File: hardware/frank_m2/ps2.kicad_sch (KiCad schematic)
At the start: 14 parts

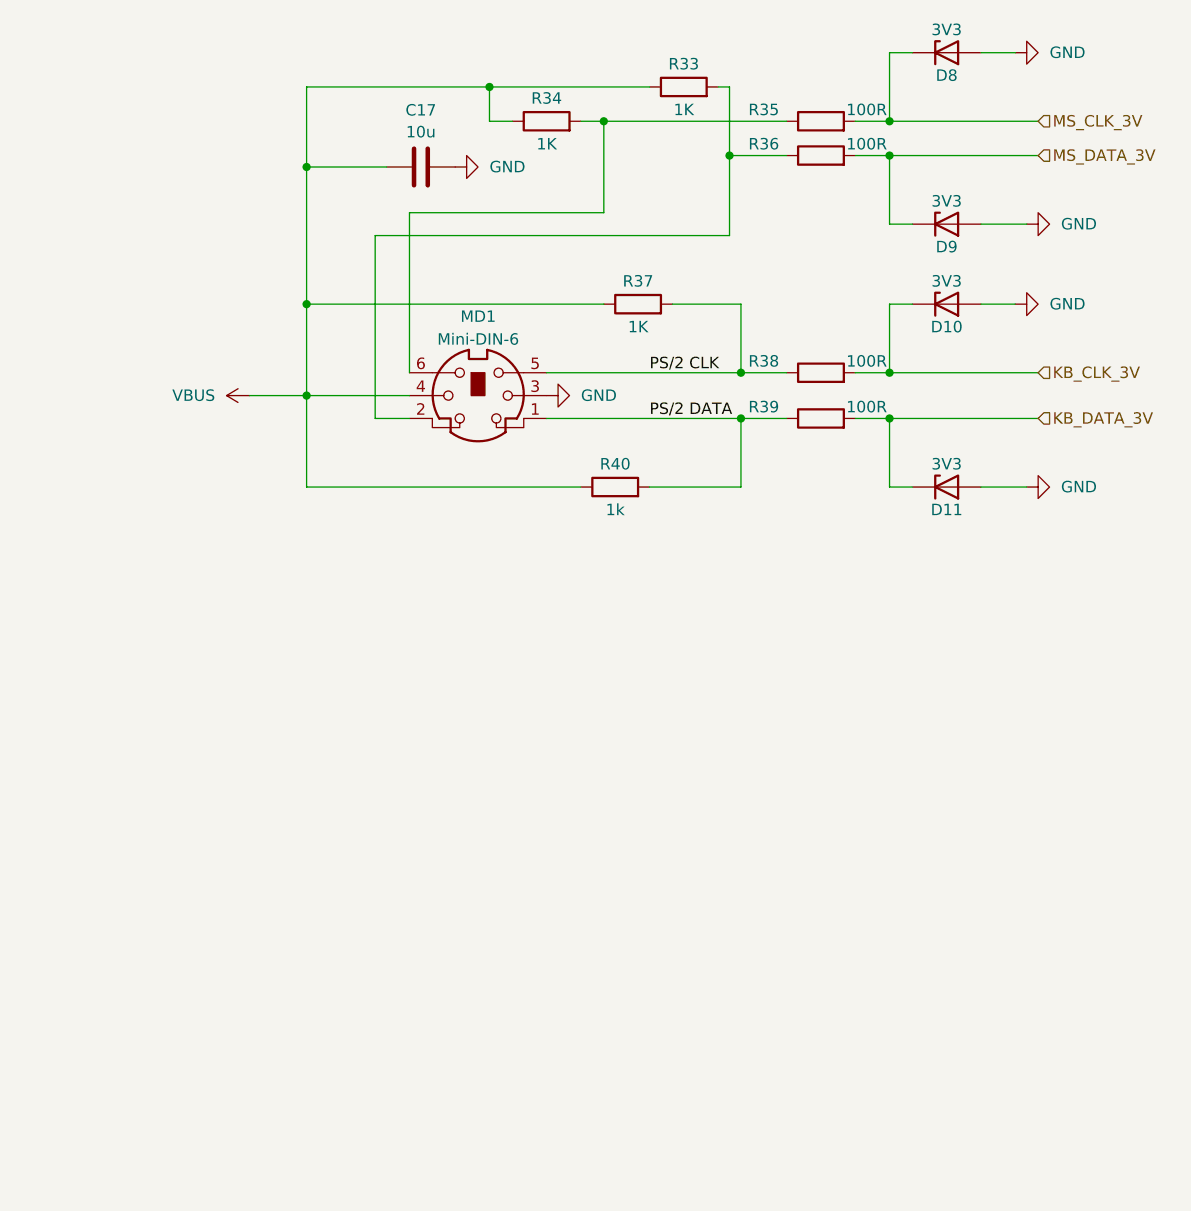
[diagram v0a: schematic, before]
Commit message: Names changed
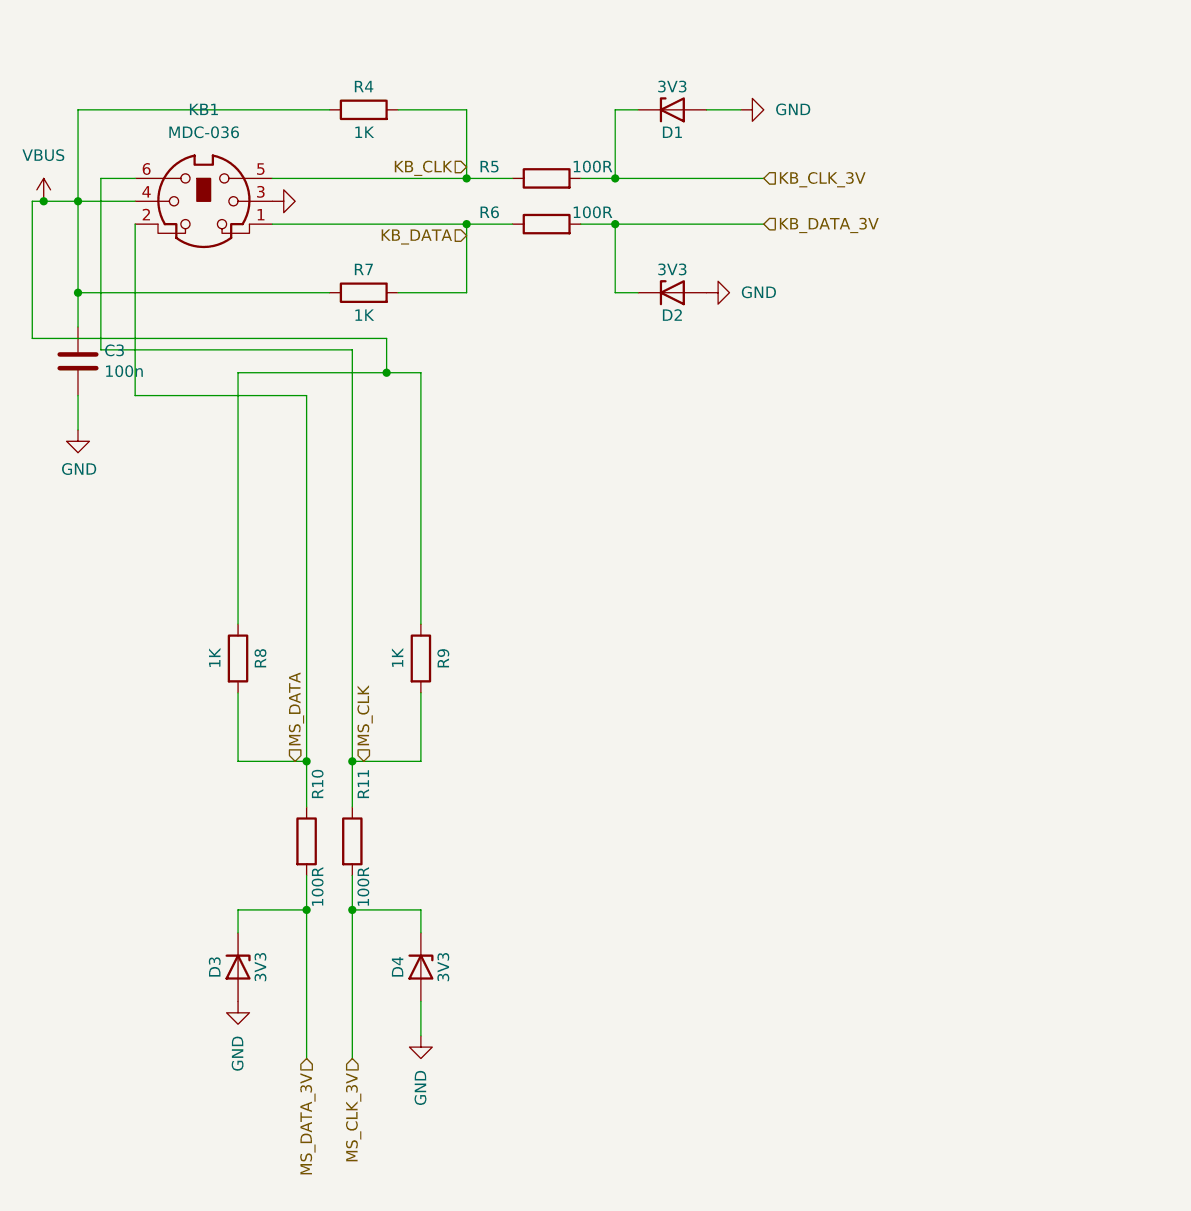
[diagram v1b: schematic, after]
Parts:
- removed C17: 10u, FRANK:Capacitor (0805), symbol Device:C
- removed D10, D11, D8, D9: 3V3, FRANK:Diode (SOD-323), symbol Device:D_Zener
- removed MD1: Mini-DIN-6, FRANK:MiniDIN (6 Pin, female), symbol Connector:Mini-DIN-6
- removed R33, R34, R37: 1K, FRANK:Resistor (0805), symbol Device:R
- removed R35, R36, R38, R39: 100R, FRANK:Resistor (0805), symbol Device:R
- removed R40: 1k, FRANK:Resistor (0805), symbol Device:R
- added C3: 100n, FRANK:Capacitor (0805), symbol Device:C
- added D1, D2, D3, D4: 3V3, FRANK:Diode (SOD-323), symbol Device:D_Zener
- added KB1: MDC-036, FRANK:MiniDIN (6 Pin, female), symbol Connector:Mini-DIN-6
- added R10, R11, R5, R6: 100R, FRANK:Resistor (0805), symbol Device:R
- added R4, R7, R8, R9: 1K, FRANK:Resistor (0805), symbol Device:R
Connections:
- net GND: now also C3.2, D1.2 (A), D2.2 (A), D3.2 (A), D4.2 (A), KB1.3
- net KB_CLK_3V: now also D1.1 (K), R5.2
- net KB_DATA_3V: now also D2.1 (K), R6.2
- net MS_CLK_3V: now also D4.1 (K), R11.2
- net MS_DATA_3V: now also D3.1 (K), R10.2
- net VBUS: now also C3.1, KB1.4, R4.1, R7.1, R8.1, R9.1
- new net KB_CLK: KB1.5, R4.2, R5.1
- new net KB_DATA: KB1.1, R6.1, R7.2
- new net MS_CLK: KB1.6, R11.1, R9.2
- new net MS_DATA: KB1.2, R10.1, R8.2
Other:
- title: Frank M2 -> FRANK

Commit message: FRANK M1 & M2 HW Revisions
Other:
- title: FRANK -> FRANK M2
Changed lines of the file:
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@@
 	(paper "A4")
 	(title_block
-		(title "FRANK")
-		(date "2025-02-18")
-		(rev "1.13")
+		(title "FRANK M2")
+		(date "2025-02-19")
+		(rev "2.1")
 		(company "Mikhail Matveev")
 		(comment 1 "https://github.com/xtremespb/frank")

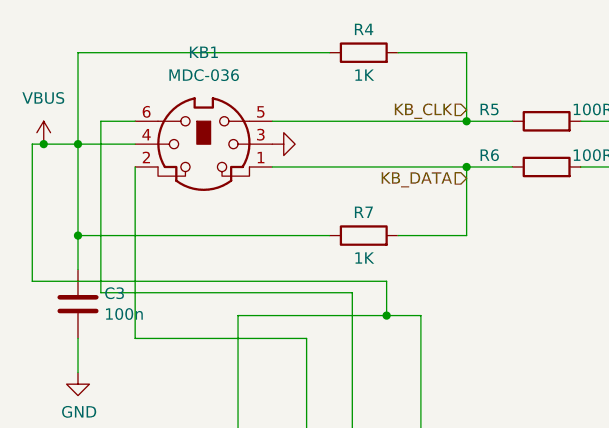
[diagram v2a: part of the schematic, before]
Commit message: HW Rev 1.02 (M2)
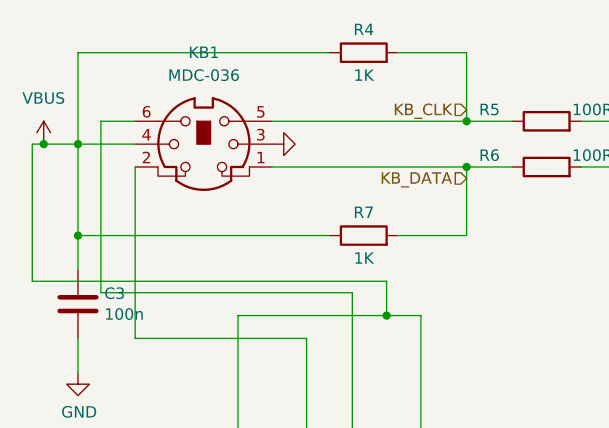
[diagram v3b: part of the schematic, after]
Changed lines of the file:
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@@
 (kicad_sch
-	(version 20231120)
+	(version 20250114)
 	(generator "eeschema")
-	(generator_version "8.0")
+	(generator_version "9.0")
 	(paper "A4")
 	(title_block
 		(title "FRANK M2")
-		(date "2025-02-19")
-		(rev "2.1")
+		(date "2025-03-04")
+		(rev "1.02")
 		(company "Mikhail Matveev")
 		(comment 1 "https://github.com/xtremespb/frank")
@@
 		(shape input)
 		(at 62.23 144.78 270)
-		(fields_autoplaced yes)
 		(effects
 			(font
@@
 		(shape input)
 		(at 63.5 111.76 90)
-		(fields_autoplaced yes)
 		(effects
 			(font
@@
 		(shape input)
 		(at 74.93 45.72 180)
-		(fields_autoplaced yes)
 		(effects
 			(font
@@
 		(shape input)
 		(at 107.95 52.07 0)
-		(fields_autoplaced yes)
 		(effects
 			(font
@@
 		(shape input)
 		(at 57.15 144.78 270)
-		(fields_autoplaced yes)
 		(effects
 			(font
@@
 		(shape input)
 		(at 55.88 111.76 90)
-		(fields_autoplaced yes)
 		(effects
 			(font
@@
 		(shape input)
 		(at 107.95 46.99 0)
-		(fields_autoplaced yes)
 		(effects
 			(font
@@
 		(shape input)
 		(at 74.93 53.34 180)
-		(fields_autoplaced yes)
 		(effects
 			(font
@@
 			)
 		)
-		(property "Description" ""
+		(property "Description" "6-pin Mini-DIN connector"
 			(at 45.72 49.53 0)
 			(effects
